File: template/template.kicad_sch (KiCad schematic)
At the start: 6 parts, among them U1 TLV62568DDC

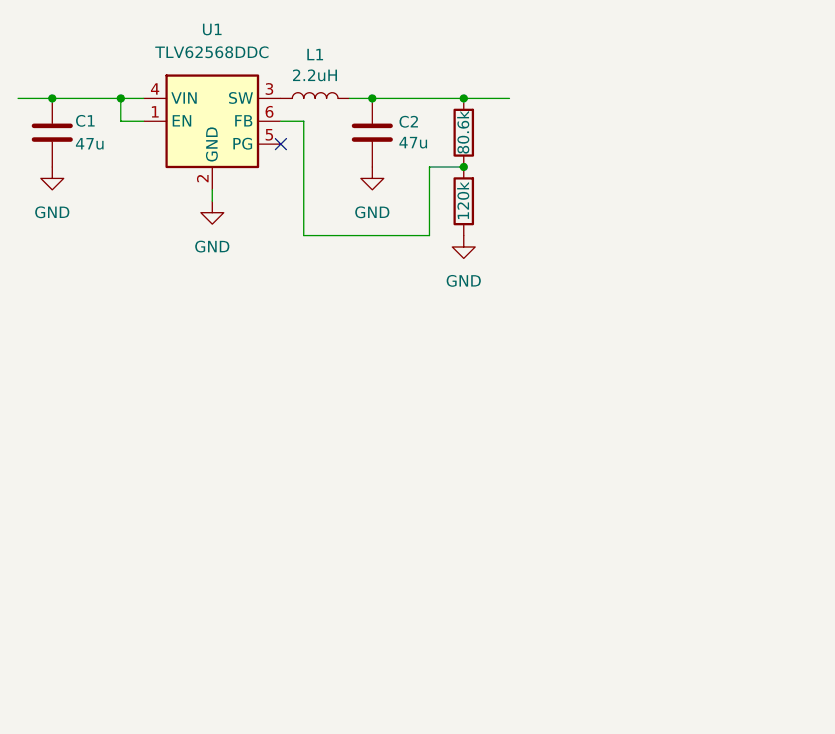
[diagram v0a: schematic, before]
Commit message: More changes
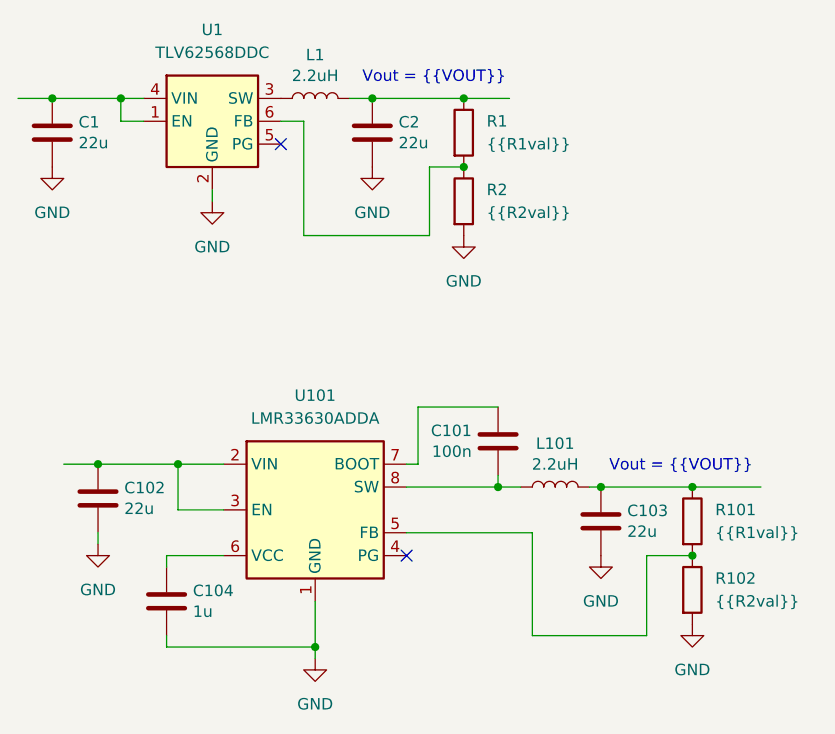
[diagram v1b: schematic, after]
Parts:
- added C101: 100n, Capacitor_SMD:C_0201_0603Metric, symbol Device:C
- added C102, C103: 22u, Capacitor_SMD:C_0603_1608Metric, symbol Device:C
- added C104: 1u, Capacitor_SMD:C_0402_1005Metric, symbol Device:C
- added L101: 2.2uH, Inductor_SMD:L_Taiyo-Yuden_NR-40xx, symbol Device:L
- added R101: {{R1val}}, Resistor_SMD:R_0402_1005Metric, symbol Device:R
- added R102: {{R2val}}, Resistor_SMD:R_0402_1005Metric, symbol Device:R
- added U101: LMR33630ADDA, Package_SO:Texas_HSOP-8-1EP_3.9x4.9mm_P1.27mm_ThermalVias, symbol Regulator_Switching:LMR33630ADDA
- C1: value 47u -> 22u; LCSC C1705 -> C59461; manf# C0805C475K9PACTU -> (none)
- C2: value 47u -> 22u; manf# C0805C226M9PACTU -> (none)
- R1: value 80.6k -> {{R1val}}; LCSC C25921 -> {{R1lcsc}}; manf# RC0805FR-07100KL -> (none)
- R2: value 120k -> {{R2val}}; LCSC C25750 -> {{R2lcsc}}; manf# RC0805FR-07120KL -> (none)
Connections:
- net GND: now also C1.2, R2.2, C102.2, C103.2, C104.2, R102.2, U101.1 (GND), U101.9 (GND); no longer C1.1, R2.1
- net at C2.1, L1.2: now also R1.1; no longer R1.2
- net at U1.1 (EN), U1.4 (VIN): now also C1.1; no longer C1.2
- new net: R1.2, R2.1, U1.6 (FB)
- new net: C103.1, L101.2, R101.1
- new net: C104.1, U101.6 (VCC)
- new net: C102.1, U101.2 (VIN), U101.3 (EN)
- new net: R101.2, R102.1, U101.5 (FB)
- new net: C101.1, U101.7 (BOOT)
- new net: C101.2, L101.1, U101.8 (SW)
- no-connect marks 1 -> 2
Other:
- note added: "Vout = {{VOUT}}"

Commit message: More updates to template
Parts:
- C101: footprint Capacitor_SMD:C_0201_0603Metric -> Capacitor_SMD:C_0402_1005Metric; LCSC C76939 -> C1525
- C102, C103: footprint Capacitor_SMD:C_0603_1608Metric -> Capacitor_SMD:C_0805_2012Metric; LCSC C59461 -> C129303
- U101: LCSC (none) -> C841384
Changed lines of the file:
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@@
 			)
 		)
-		(property "Footprint" "Capacitor_SMD:C_0603_1608Metric"
+		(property "Footprint" "Capacitor_SMD:C_0805_2012Metric"
 			(at 103.8352 87.63 0)
 			(effects
@@
 			)
 		)
-		(property "LCSC" "C59461"
+		(property "LCSC" "C129303"
 			(at 102.87 83.82 0)
 			(effects
@@
 			)
 		)
-		(property "Footprint" "Capacitor_SMD:C_0603_1608Metric"
+		(property "Footprint" "Capacitor_SMD:C_0805_2012Metric"
 			(at 47.9552 85.09 0)
 			(effects
@@
 			)
 		)
-		(property "LCSC" "C59461"
+		(property "LCSC" "C129303"
 			(at 46.99 81.28 0)
 			(effects
@@
 			)
 		)
-		(property "Footprint" "Capacitor_SMD:C_0201_0603Metric"
+		(property "Footprint" "Capacitor_SMD:C_0402_1005Metric"
 			(at 90.4748 78.74 0)
 			(effects
@@
 			)
 		)
-		(property "LCSC" "C76939"
+		(property "LCSC" "C1525"
 			(at 91.44 74.93 0)
 			(effects
@@
 			(at 71.12 82.55 0)
 			(effects
+				(font
+					(size 1.27 1.27)
+				)
+				(hide yes)
+			)
+		)
+		(property "LCSC" "C841384"
+			(at 71.12 82.55 0)
+			(effects
